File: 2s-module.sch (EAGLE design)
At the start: 3 parts, among them J1 CQ-USB-C16PSMT01

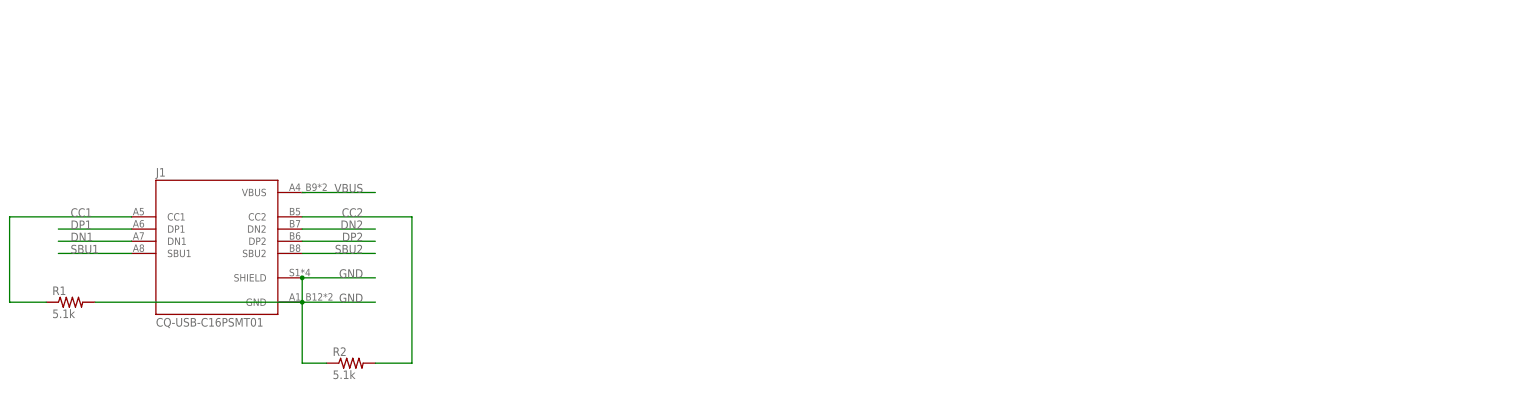
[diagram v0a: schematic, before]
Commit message: build balancer prototype
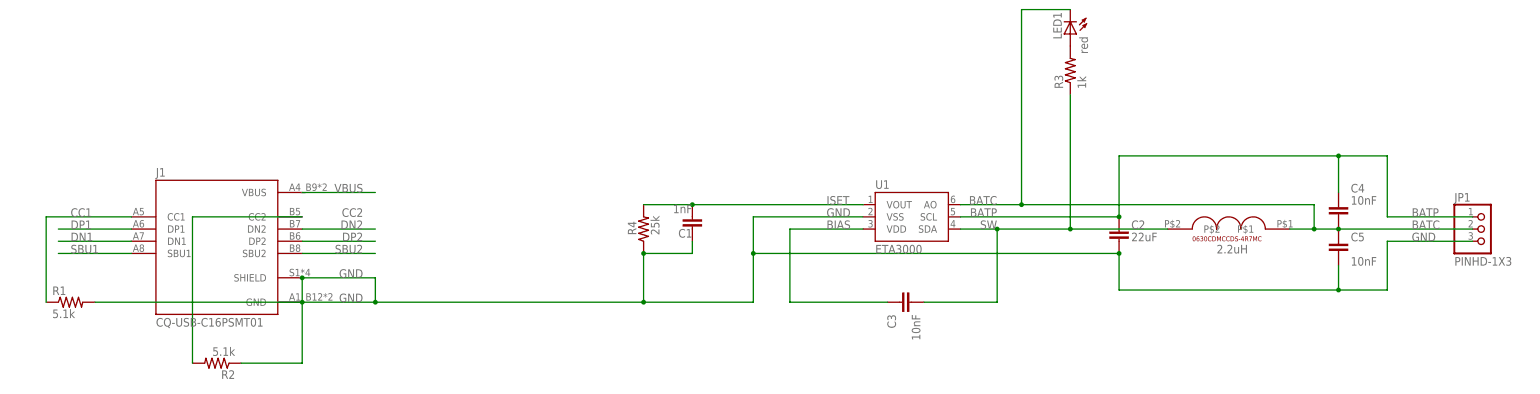
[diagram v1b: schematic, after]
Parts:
- added C1: 1nF, Capacitor:C_CHIP-0603(1608-METRIC)
- added C2: 22uF, Capacitor:C_CHIP-1206(3216-METRIC)
- added C3, C4, C5: 10nF, Capacitor:C_CHIP-0603(1608-METRIC)
- added JP1: PINHD-1X3, Connector:PINHD-1X3
- added L1: 0630CDMCCDS-4R7MC, 0630CDMCCDS-4R7MC:0630CDMCCDS-4R7MC
- added LED1: red, adafruit:LEDCHIPLED_0603
- added R3: 1k, resistor:R-US_R0603
- added R4: 25k, resistor:R-US_R0603
- added U1: MCP4725, SparkFun-IC-Conversion:MCP4725SOT-23
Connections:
- new net BATC: C4.2, C5.1, JP1.2, L1.P$1, LED1.C, U1.AO
- new net BATP: C2.1, C4.1, JP1.1, U1.SCL
- new net BIAS: C3.2, U1.VDD
- new net ISET: C1.2, R4.2, U1.VOUT
- new net N$1: LED1.A, R3.2
- new net SW: C3.1, L1.P$2, R3.1, U1.SDA
- net GND: now also C1.1, C2.2, C5.2, JP1.3, R4.1, U1.VSS
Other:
- note added: "2.2uH"
- note added: "ETA3000"
- moved on the sheet: R2
